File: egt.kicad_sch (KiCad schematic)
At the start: 9 parts, among them U4 MAX31855KASA

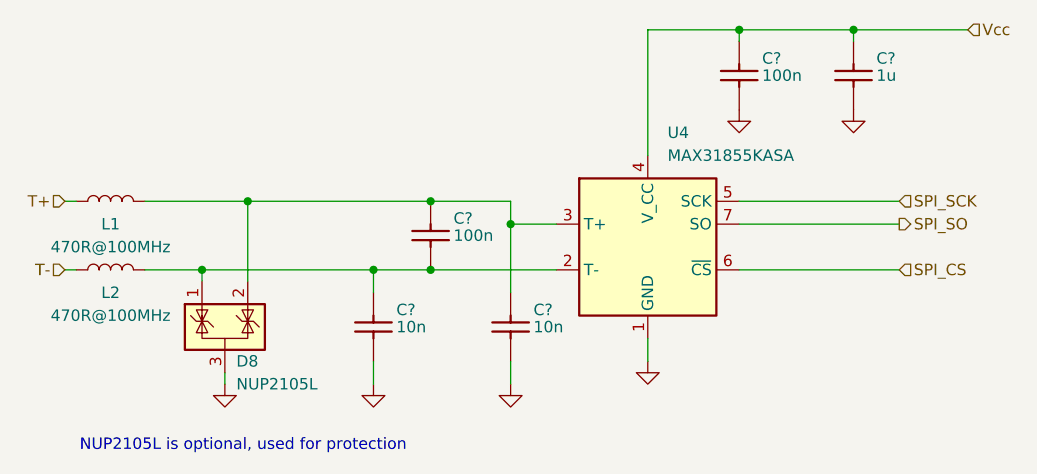
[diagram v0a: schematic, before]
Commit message: Unification with UAEFI F7 #114 #110
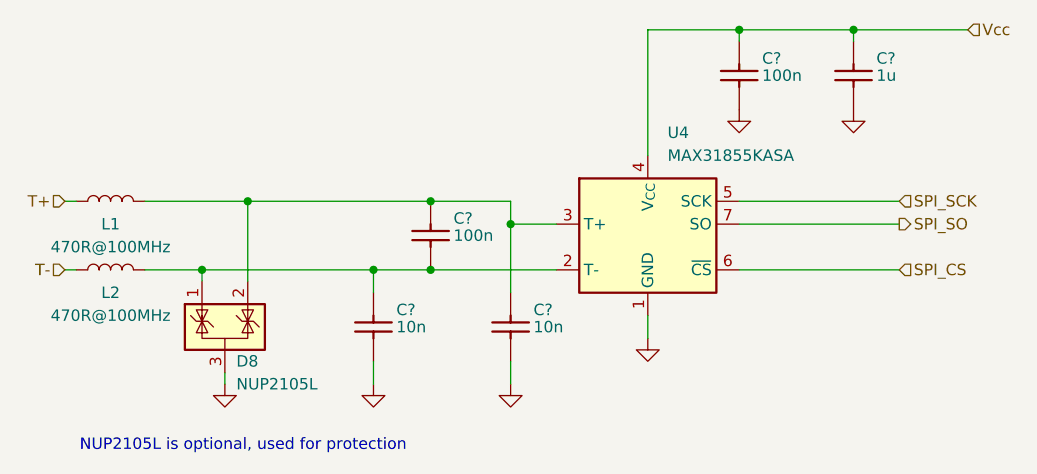
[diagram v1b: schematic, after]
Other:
- moved on the sheet: U4
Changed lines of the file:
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@@
 	(title_block
 		(title "UAEFI")
-		(date "2025-04-30")
-		(rev "E")
+		(date "2026-07-05")
+		(rev "F")
 		(company "rusEFI.com")
 	)
@@
 	(wire
 		(pts
-			(xy 166.37 102.87) (xy 166.37 105.41)
+			(xy 166.37 100.33) (xy 166.37 102.87)
 		)
 		(stroke
@@
 	)
 	(symbol
-		(lib_name "MAX31855KASA_1")
 		(lib_id "Sensor_Temperature:MAX31855KASA")
 		(at 166.37 92.71 0)
@@
 			)
 		)
-		(property "Description" ""
+		(property "Description" "Cold Junction K-type Thermocouple Interface, SPI, SOIC-8"
 			(at 166.37 92.71 0)
 			(effects
@@
 		)
 		(pin "7"
+		)
+		(pin "8"
 		)
 		(instances
@@
 			)
 		)
-		(property "Datasheet" "http://www.onsemi.com/pub_link/Collateral/NUP2105L-D.PDF"
+		(property "Datasheet" "https://www.onsemi.com/pub_link/Collateral/NUP2105L-D.PDF"
 			(at 122.555 98.425 0)
 			(effects
@@
 			)
 		)
-		(property "Description" ""
+		(property "Description" "Dual Line CAN Bus Protector, 24Vrwm"
 			(at 119.38 101.6 0)
 			(effects
@@
 	(symbol
 		(lib_id "power:GND")
-		(at 166.37 105.41 0)
+		(at 166.37 102.87 0)
 		(unit 1)
 		(exclude_from_sim no)
@@
 		(dnp no)
 		(property "Reference" "#PWR0108"
-			(at 166.37 111.76 0)
+			(at 166.37 109.22 0)
 			(effects
 				(font
@@
 		)
 		(property "Value" "GND"
-			(at 166.497 109.8042 0)
+			(at 166.497 107.2642 0)
 			(effects
 				(font
@@
 		)
 		(property "Footprint" ""
-			(at 166.37 105.41 0)
+			(at 166.37 102.87 0)
 			(effects
 				(font
@@
 		)
 		(property "Datasheet" ""
-			(at 166.37 105.41 0)
+			(at 166.37 102.87 0)
 			(effects
 				(font
@@
 		)
 		(property "Description" "Power symbol creates a global label with name \"GND\" , ground"
-			(at 166.37 105.41 0)
-			(effects
-				(font
+			(at 166.37 102.87 0)
+			(effects
+				(font
